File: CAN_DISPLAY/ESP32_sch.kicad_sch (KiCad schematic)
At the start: 37 parts, among them J10 Prodrammer, J11 Micro_SD_Card, J12 J-Link, J15 LED Display, SW1 BOOT, SW2 RESET, U1 ESP32-DevKit, U2 ESP32-WROOM-E

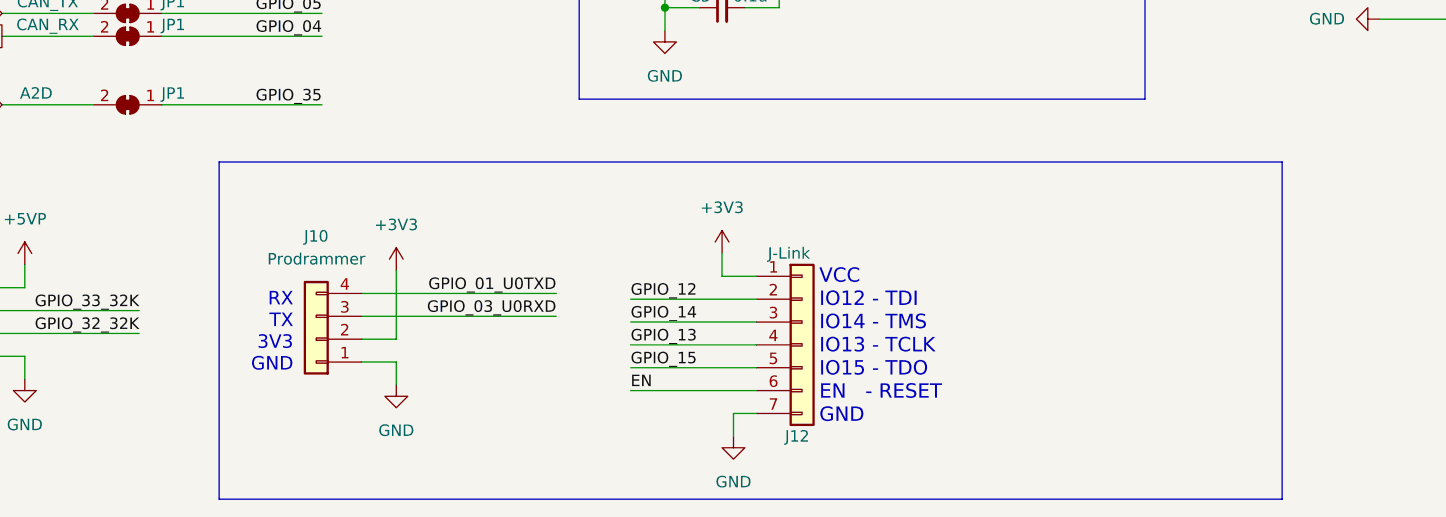
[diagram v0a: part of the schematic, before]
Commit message: PCB Fixes
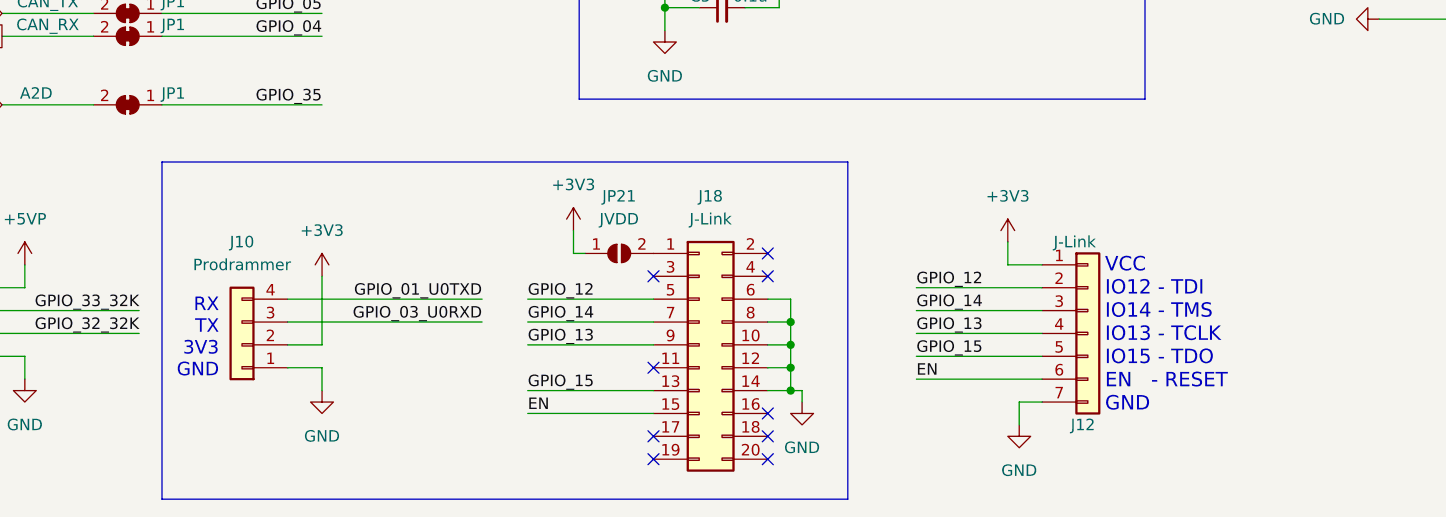
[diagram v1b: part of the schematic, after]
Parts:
- added J18: J-Link, Connector_PinHeader_2.54mm:PinHeader_2x10_P2.54mm_Vertical, symbol Connector_Generic:Conn_02x10_Odd_Even
- added JP21: JVDD, Jumper:SolderJumper-2_P1.3mm_Open_RoundedPad1.0x1.5mm, symbol Jumper:SolderJumper_2_Open
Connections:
- net +3V3: now also JP21.1 (A)
- net EN: now also J18.15 (Pin_15)
- net GND: now also J18.10 (Pin_10), J18.12 (Pin_12), J18.14 (Pin_14), J18.6 (Pin_6), J18.8 (Pin_8)
- net GPIO_12: now also J18.5 (Pin_5)
- net GPIO_13: now also J18.9 (Pin_9)
- net GPIO_14: now also J18.7 (Pin_7)
- net GPIO_15: now also J18.13 (Pin_13)
- new net: J18.1 (Pin_1), JP21.2 (B)
- no-connect marks 6 -> 15
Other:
- moved on the sheet: J10, J12
